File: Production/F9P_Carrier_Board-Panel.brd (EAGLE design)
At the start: 155.7 x 146.3 mm, 666 parts, among them J11 MICROMOD-2222-C, J13 U.FL, J14 QWIIC_RIGHT_ANGLE, J17 JTAG, J20 MICROMOD-2222-C, J22 U.FL, J23 QWIIC_RIGHT_ANGLE, J26 JTAG, J29 MICROMOD-2222-C, J31 U.FL, J32 QWIIC_RIGHT_ANGLE, J35 JTAG, J4 U.FL, J5 QWIIC_RIGHT_ANGLE, J6 MICROMOD-2222-C, J8 JTAG, U1 U-BLOX_ZED-F9P, U2 AP7361C-33, U3 U-BLOX_ZED-F9P, U4 AP7361C-33, U5 AP7361C-33, U6 U-BLOX_ZED-F9P, U7 AP7361C-33, U8 U-BLOX_ZED-F9P

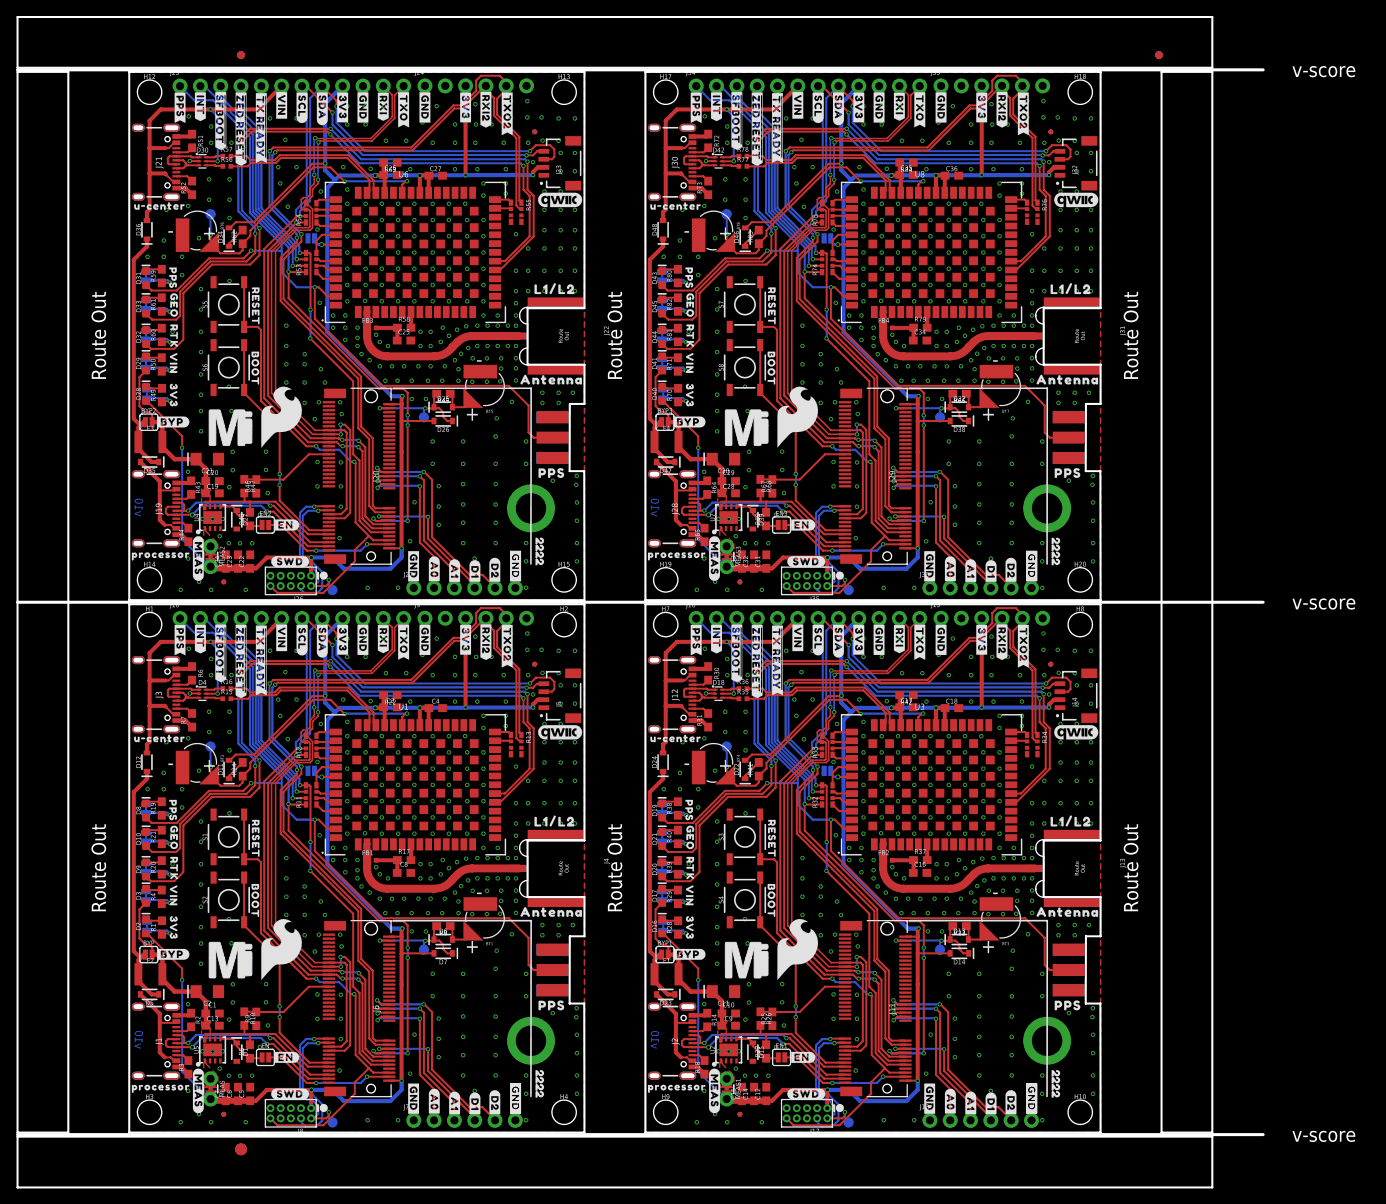
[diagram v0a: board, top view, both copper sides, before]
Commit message: Updated panel
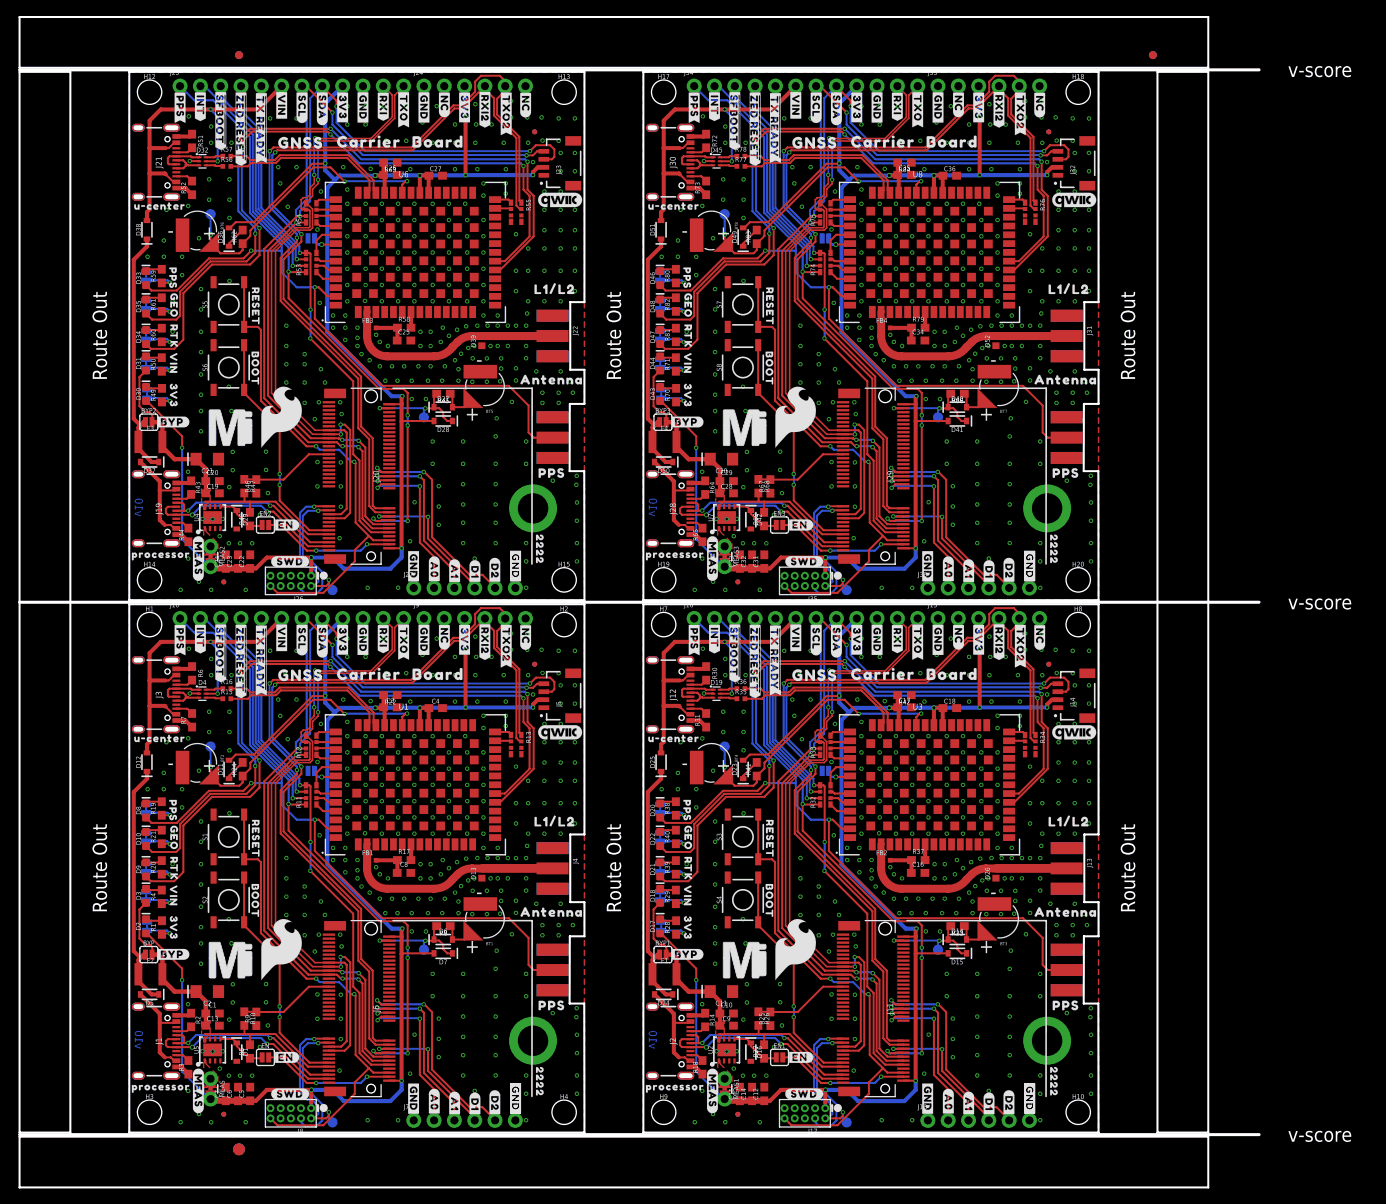
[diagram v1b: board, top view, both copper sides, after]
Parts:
- added D49: 0.5A/40V/420mV, SparkFun-DiscreteSemi:SOD-323
- added D50, D51: 3A/10V/280mV, SparkFun-DiscreteSemi:SOD-323
- added D52: PESD0402, SparkFun-DiscreteSemi:0402
- added U$329: (no value), bot:##SFBOOT##8
- added U$330: (no value), SparkFun-MicroMod:MICROMOD_LOGO_.5
- added U$331: (no value), SparkFun-MicroMod:MICROMOD_MI_LOGO_1
- added U$332: (no value), SparkFun-Aesthetics:SFE_LOGO_FLAME_.3
- added U$333, U$334, U$335, U$346, U$347: (no value), top:#GND#0
- added U$336: (no value), top:#A0#8
- added U$337: (no value), top:#A1#8
- added U$338: (no value), top:#D1#8
- added U$339: (no value), top:#D2#8
- added U$340, U$341: (no value), top:PROCESSOR23
- added U$342: (no value), bot:#A0#14
- added U$343: (no value), bot:#A1#14
- added U$344: (no value), bot:#D1#14
- added U$345: (no value), bot:#D2#14
- added U$348: (no value), top:GNSS21
- added U$349: (no value), top:GNSS501
- added U$350: (no value), top:CARRIER502
- added U$351: (no value), top:BOARD503
- added U$352: (no value), top:2222501
- added U$353, U$354: (no value), top:#NC#4
- added U$355, U$356: (no value), top:#NC#5
- D13: value 3A/10V/280mV -> PESD0402; device SparkFun-DiscreteSemi:SOD-323 -> SparkFun-DiscreteSemi:0402
- D14, D38: value 1A/23V/620mV -> 3A/10V/280mV
- D15: value 3.3V -> 1A/23V/620mV
- D16, D29: value RED -> 3.3V; device SparkFun-LED:LED-0603 -> SparkFun-DiscreteSemi:SOD-323
- D18, D30: value PRTR5V0U2F -> RED; device SparkFun-IC-Power:SOT886 -> SparkFun-LED:LED-0603
- D19, D32, D45: value BLUE -> PRTR5V0U2F; device SparkFun-LED:LED-0603 -> SparkFun-IC-Power:SOT886
- D22, D34, D46: value 0.5A/40V/420mV -> BLUE; device SparkFun-DiscreteSemi:SOD-323 -> SparkFun-LED:LED-0603
- D23, D36: value 3A/10V/280mV -> 0.5A/40V/420mV
- D26: value 1A/23V/620mV -> PESD0402; device SparkFun-DiscreteSemi:SOD-323 -> SparkFun-DiscreteSemi:0402
- D27: value 3.3V -> 3A/10V/280mV
- D28, D41: value RED -> 1A/23V/620mV; device SparkFun-LED:LED-0603 -> SparkFun-DiscreteSemi:SOD-323
- D31, D43, D44: value BLUE -> RED
- D35, D47, D48: value 3A/10V/280mV -> BLUE; device SparkFun-DiscreteSemi:SOD-323 -> SparkFun-LED:LED-0603
- D39: value 3.3V -> PESD0402; device SparkFun-DiscreteSemi:SOD-323 -> SparkFun-DiscreteSemi:0402
- D40: value RED -> 3A/10V/280mV; device SparkFun-LED:LED-0603 -> SparkFun-DiscreteSemi:SOD-323
- D42: value PRTR5V0U2F -> 3.3V; device SparkFun-IC-Power:SOT886 -> SparkFun-DiscreteSemi:SOD-323
- H11, H16, H5, H6: value STAND-OFF-REFLOW2.5MM_TALL -> STAND-OFF-REFLOW-M2.5_2.5MM_TALL
- J13, J22, J31, J4: device SparkFun-RF:SMA-EDGE-SMD -> SparkFun-RF:SMA-EDGE
- MEAS, MEAS1, MEAS2, MEAS3: value (none) -> JUMPER-COMBO_2_NC_TRACE
- U$100: device top:GEO15 -> top:#GND#0
- U$101: device top:PPS14 -> top:#GND#0
- U$102: device top:RTK16 -> top:#PPS#6
- U$103: device bot:#GEO#9 -> top:#RXI2#9
- U$104: device bot:#PPS#10 -> top:#TXO2#9
- U$105: device bot:#RTK#8 -> top:#VIN#13
- U$106: device bot:#SPI#11 -> top:GEO15
- U$107: device top:#3V3#1 -> top:PPS14
- U$108: device top:#3V3#1 -> top:RTK16
- U$109: device top:#GND#0 -> bot:#GEO#9
- U$110: device top:#GND#0 -> bot:#PPS#10
- U$111: device top:#VIN#13 -> bot:#RTK#8
- U$112: device top:#INT#10 -> bot:#SPI#11
- U$113, U$281: device top:##TX_READY##13 -> top:#3V3#1
- U$114: device bot:##TX_READY##7 -> top:#3V3#1
- U$115, U$283: device bot:#INT#4 -> top:#GND#0
- U$116: device bot:#PPS#3 -> top:#GND#0
- U$117: device bot:#TXO2#10 -> top:#VIN#13
- U$118: device bot:#RXI2#10 -> top:#INT#10
- U$119: device top:ZED#F9P19 -> top:##TX_READY##13
- U$120: device top:U#CENTER20 -> bot:##TX_READY##7
- U$121: device SparkFun-Aesthetics:QWIIC_5.5MM -> bot:#INT#4
- U$122: device bot:#SCL#1 -> bot:#PPS#3
- U$123: device bot:#SDA#0 -> bot:#TXO2#10
- U$124: device bot:#TXO#5 -> bot:#RXI2#10
- U$125: device bot:#RXI#6 -> top:ZED#F9P19
- U$126: device top:PPS15 -> top:U#CENTER20
- U$127: device top:ANTENNA16 -> SparkFun-Aesthetics:QWIIC_5.5MM
- U$128: device top:L1#L216 -> bot:#SCL#1
- U$129: device top:##CS##9 -> bot:#SDA#0
- U$130: device top:#CLK#7 -> bot:#TXO#5
- U$135: device top:#SDO#9 -> bot:#RXI#6
- U$136: device top:#SDI#11 -> top:PPS15
- U$137: device top:BLUETOOTH24 -> top:ANTENNA16
- U$138: device top:U#CENTER22 -> top:L1#L216
- U$139: device top:L1#L217 -> top:##CS##9
- U$140: device top:ANTENNA17 -> top:#CLK#7
- U$141: device top:PPS16 -> top:#SDO#9
- U$142: device bot:##ZED_RESET##9 -> top:#SDI#11
- U$143: device top:##ZED_RESET##14 -> top:BLUETOOTH24
- U$144: device top:##SFBOOT##13 -> top:U#CENTER22
- U$145: device bot:##SFBOOT##8 -> top:L1#L217
- U$146: device SparkFun-MicroMod:MICROMOD_LOGO_.5 -> top:ANTENNA17
- U$147: device SparkFun-MicroMod:MICROMOD_MI_LOGO_1 -> top:PPS16
- U$148: device SparkFun-Aesthetics:SFE_LOGO_FLAME_.3 -> bot:##ZED_RESET##9
- U$149, U$327: device top:#GND#0 -> top:##ZED_RESET##14
- U$150: device top:#GND#0 -> top:##SFBOOT##13
- U$151: device top:#GND#0 -> bot:##SFBOOT##8
- U$152: device top:#A0#8 -> SparkFun-MicroMod:MICROMOD_LOGO_.5
- U$153: device top:#A1#8 -> SparkFun-MicroMod:MICROMOD_MI_LOGO_1
- U$154: device top:#D1#8 -> SparkFun-Aesthetics:SFE_LOGO_FLAME_.3
- U$155: device top:#D2#8 -> top:#GND#0
- U$156, U$157: device top:PROCESSOR23 -> top:#GND#0
- U$158: device bot:#A0#14 -> top:#A0#8
- U$159: device bot:#A1#14 -> top:#A1#8
- U$160: device bot:#D1#14 -> top:#D1#8
- U$161: device bot:#D2#14 -> top:#D2#8
- U$162, U$163: device top:#GND#0 -> top:PROCESSOR23
- U$164: device top:GNSS21 -> bot:#A0#14
- U$165: device buzzard_labels (9):22229 -> bot:#A1#14
- U$166: device power:#BYP#8 -> bot:#D1#14
- U$167: device power:#RESET10 -> bot:#D2#14
- U$168: device power:BOOT10 -> top:#GND#0
- U$169: device power:#MEAS#10 -> top:#GND#0
- U$170: device power:#SWD#10 -> top:GNSS21
- U$171: device headers_dup:VIN3 -> top:GNSS501
- U$172: device headers_dup:3V34 -> top:CARRIER502
- U$173: device fl3:#SWD#10 -> top:BOARD503
- U$174: device fl3:#MEAS#10 -> top:2222501
- U$175: device fl3:#VIN_LED#10 -> top:#NC#4
- U$176: device fl3:#3V3_LED#10 -> top:#NC#4
- U$177: device output:#EN#0 -> top:#NC#5
- U$178: device top:#3V3#1 -> top:#NC#5
- U$179: device top:#3V3#1 -> power:#BYP#8
- U$180: device top:#GND#0 -> power:#RESET10
- U$181: device top:#GND#0 -> power:BOOT10
- U$182: device top:#PPS#6 -> power:#MEAS#10
- U$183: device top:#RXI2#9 -> power:#SWD#10
- U$184: device top:#TXO2#9 -> headers_dup:VIN3
- U$185: device top:#VIN#13 -> headers_dup:3V34
- U$186: device top:GEO15 -> fl3:#SWD#10
- U$187: device top:PPS14 -> fl3:#MEAS#10
- U$188: device top:RTK16 -> fl3:#VIN_LED#10
- U$189: device bot:#GEO#9 -> fl3:#3V3_LED#10
- U$190: device bot:#PPS#10 -> output:#EN#0
- U$191: device bot:#RTK#8 -> top:#3V3#1
- U$192: device bot:#SPI#11 -> top:#3V3#1
- U$193, U$194: device top:#3V3#1 -> top:#GND#0
- U$195: device top:#GND#0 -> top:#PPS#6
- U$196: device top:#GND#0 -> top:#RXI2#9
- U$197: device top:#VIN#13 -> top:#TXO2#9
- U$198: device top:#INT#10 -> top:#VIN#13
- U$199: device top:##TX_READY##13 -> top:GEO15
- U$200: device bot:##TX_READY##7 -> top:PPS14
- U$201: device bot:#INT#4 -> top:RTK16
- U$202: device bot:#PPS#3 -> bot:#GEO#9
- U$203: device bot:#TXO2#10 -> bot:#PPS#10
- U$204: device bot:#RXI2#10 -> bot:#RTK#8
- U$205: device top:ZED#F9P19 -> bot:#SPI#11
- U$206: device top:U#CENTER20 -> top:#3V3#1
- U$207: device SparkFun-Aesthetics:QWIIC_5.5MM -> top:#3V3#1
- U$208: device bot:#SCL#1 -> top:#GND#0
- U$209: device bot:#SDA#0 -> top:#GND#0
- U$210: device bot:#TXO#5 -> top:#VIN#13
- U$211: device bot:#RXI#6 -> top:#INT#10
- U$212: device top:PPS15 -> top:##TX_READY##13
- U$213: device top:ANTENNA16 -> bot:##TX_READY##7
- U$214: device top:L1#L216 -> bot:#INT#4
- U$215: device top:##CS##9 -> bot:#PPS#3
- U$216: device top:#CLK#7 -> bot:#TXO2#10
- U$217: device top:#SDO#9 -> bot:#RXI2#10
- U$218: device top:#SDI#11 -> top:ZED#F9P19
- U$219: device top:BLUETOOTH24 -> top:U#CENTER20
- U$220: device top:U#CENTER22 -> SparkFun-Aesthetics:QWIIC_5.5MM
- U$221: device top:L1#L217 -> bot:#SCL#1
- U$222: device top:ANTENNA17 -> bot:#SDA#0
- U$223: device top:PPS16 -> bot:#TXO#5
- U$224: device bot:##ZED_RESET##9 -> bot:#RXI#6
- U$225: device top:##ZED_RESET##14 -> top:PPS15
- U$226: device top:##SFBOOT##13 -> top:ANTENNA16
- U$227: device bot:##SFBOOT##8 -> top:L1#L216
- U$228: device SparkFun-MicroMod:MICROMOD_LOGO_.5 -> top:##CS##9
- U$229: device SparkFun-MicroMod:MICROMOD_MI_LOGO_1 -> top:#CLK#7
- U$230: device SparkFun-Aesthetics:SFE_LOGO_FLAME_.3 -> top:#SDO#9
- U$231: device top:#GND#0 -> top:#SDI#11
- U$232: device top:#GND#0 -> top:BLUETOOTH24
- U$233: device top:#GND#0 -> top:U#CENTER22
- U$234: device top:#A0#8 -> top:L1#L217
- U$235: device top:#A1#8 -> top:ANTENNA17
- U$236: device top:#D1#8 -> top:PPS16
- U$237: device top:#D2#8 -> bot:##ZED_RESET##9
- U$238: device top:PROCESSOR23 -> top:##ZED_RESET##14
- U$239: device top:PROCESSOR23 -> top:##SFBOOT##13
- U$240: device bot:#A0#14 -> bot:##SFBOOT##8
- U$241: device bot:#A1#14 -> SparkFun-MicroMod:MICROMOD_LOGO_.5
- U$242: device bot:#D1#14 -> SparkFun-MicroMod:MICROMOD_MI_LOGO_1
- U$243: device bot:#D2#14 -> SparkFun-Aesthetics:SFE_LOGO_FLAME_.3
- U$246: device top:GNSS21 -> top:#GND#0
- U$247: device buzzard_labels (9):22229 -> top:#A0#8
- U$248: device power:#BYP#8 -> top:#A1#8
- U$249: device power:#RESET10 -> top:#D1#8
- U$250: device power:BOOT10 -> top:#D2#8
- U$251: device power:#MEAS#10 -> top:PROCESSOR23
- U$252: device power:#SWD#10 -> top:PROCESSOR23
- U$253: device headers_dup:VIN3 -> bot:#A0#14
- U$254: device headers_dup:3V34 -> bot:#A1#14
- U$255: device fl3:#SWD#10 -> bot:#D1#14
- U$256: device fl3:#MEAS#10 -> bot:#D2#14
- U$257: device fl3:#VIN_LED#10 -> top:#GND#0
- U$258: device fl3:#3V3_LED#10 -> top:#GND#0
- U$259: device output:#EN#0 -> top:GNSS21
- U$260: device top:#3V3#1 -> top:GNSS501
- U$261: device top:#3V3#1 -> top:CARRIER502
- U$262: device top:#GND#0 -> top:BOARD503
- U$263: device top:#GND#0 -> top:2222501
- U$264: device top:#PPS#6 -> top:#NC#4
- U$265: device top:#RXI2#9 -> top:#NC#4
- U$266: device top:#TXO2#9 -> top:#NC#5
- U$267: device top:#VIN#13 -> top:#NC#5
- U$268: device top:GEO15 -> power:#BYP#8
- U$269: device top:PPS14 -> power:#RESET10
- U$270: device top:RTK16 -> power:BOOT10
- U$271: device bot:#GEO#9 -> power:#MEAS#10
- U$272: device bot:#PPS#10 -> power:#SWD#10
- U$273: device bot:#RTK#8 -> headers_dup:VIN3
- U$274: device bot:#SPI#11 -> headers_dup:3V34
- U$275, U$93: device top:#3V3#1 -> fl3:#SWD#10
- U$276: device top:#3V3#1 -> fl3:#MEAS#10
- U$277, U$95: device top:#GND#0 -> fl3:#VIN_LED#10
- U$278: device top:#GND#0 -> fl3:#3V3_LED#10
- U$279: device top:#VIN#13 -> output:#EN#0
- U$280: device top:#INT#10 -> top:#3V3#1
- U$282: device bot:##TX_READY##7 -> top:#GND#0
- U$284: device bot:#PPS#3 -> top:#PPS#6
- U$285: device bot:#TXO2#10 -> top:#RXI2#9
- U$286: device bot:#RXI2#10 -> top:#TXO2#9
- U$287: device top:ZED#F9P19 -> top:#VIN#13
- U$288: device top:U#CENTER20 -> top:GEO15
- U$289: device SparkFun-Aesthetics:QWIIC_5.5MM -> top:PPS14
- U$290: device bot:#SCL#1 -> top:RTK16
- U$291: device bot:#SDA#0 -> bot:#GEO#9
- U$292: device bot:#TXO#5 -> bot:#PPS#10
- U$293: device bot:#RXI#6 -> bot:#RTK#8
- U$294: device top:PPS15 -> bot:#SPI#11
- U$295: device top:ANTENNA16 -> top:#3V3#1
- U$296: device top:L1#L216 -> top:#3V3#1
- U$297: device top:##CS##9 -> top:#GND#0
- U$298: device top:#CLK#7 -> top:#GND#0
- U$299: device top:#SDO#9 -> top:#VIN#13
- U$300: device top:#SDI#11 -> top:#INT#10
- U$301: device top:BLUETOOTH24 -> top:##TX_READY##13
- U$302: device top:U#CENTER22 -> bot:##TX_READY##7
- U$303: device top:L1#L217 -> bot:#INT#4
- U$304: device top:ANTENNA17 -> bot:#PPS#3
- U$305: device top:PPS16 -> bot:#TXO2#10
- U$306: device bot:##ZED_RESET##9 -> bot:#RXI2#10
- U$307: device top:##ZED_RESET##14 -> top:ZED#F9P19
- U$308: device top:##SFBOOT##13 -> top:U#CENTER20
- U$309: device bot:##SFBOOT##8 -> SparkFun-Aesthetics:QWIIC_5.5MM
- U$310: device SparkFun-MicroMod:MICROMOD_LOGO_.5 -> bot:#SCL#1
- U$311: device SparkFun-MicroMod:MICROMOD_MI_LOGO_1 -> bot:#SDA#0
- U$312: device SparkFun-Aesthetics:SFE_LOGO_FLAME_.3 -> bot:#TXO#5
- U$313: device top:#GND#0 -> bot:#RXI#6
- U$314: device top:#GND#0 -> top:PPS15
- U$315: device top:#GND#0 -> top:ANTENNA16
- U$316: device top:#A0#8 -> top:L1#L216
- U$317: device top:#A1#8 -> top:##CS##9
- U$318: device top:#D1#8 -> top:#CLK#7
- U$319: device top:#D2#8 -> top:#SDO#9
- U$320: device top:PROCESSOR23 -> top:#SDI#11
- U$321: device top:PROCESSOR23 -> top:BLUETOOTH24
- U$322: device bot:#A0#14 -> top:U#CENTER22
- U$323: device bot:#A1#14 -> top:L1#L217
- U$324: device bot:#D1#14 -> top:ANTENNA17
- U$325: device bot:#D2#14 -> top:PPS16
- U$326: device top:#GND#0 -> bot:##ZED_RESET##9
- U$328: device top:GNSS21 -> top:##SFBOOT##13
- U$55: device buzzard_labels (9):22229 -> top:#NC#4
- U$79: device buzzard_labels (9):22229 -> top:GNSS501
- U$80: device power:#BYP#8 -> top:CARRIER502
- U$81: device power:#RESET10 -> top:BOARD503
- U$82: device power:BOOT10 -> top:2222501
- U$83: device power:#MEAS#10 -> top:#NC#4
- U$84: device power:#SWD#10 -> top:#NC#5
- U$85: device headers_dup:VIN3 -> top:#NC#5
- U$86: device headers_dup:3V34 -> power:#BYP#8
- U$87: device fl3:#SWD#10 -> power:#RESET10
- U$88: device fl3:#MEAS#10 -> power:BOOT10
- U$89: device fl3:#VIN_LED#10 -> power:#MEAS#10
- U$90: device fl3:#3V3_LED#10 -> power:#SWD#10
- U$91: device output:#EN#0 -> headers_dup:VIN3
- U$92: device top:#3V3#1 -> headers_dup:3V34
- U$94: device top:#GND#0 -> fl3:#MEAS#10
- U$96: device top:#PPS#6 -> fl3:#3V3_LED#10
- U$97: device top:#RXI2#9 -> output:#EN#0
- U$98: device top:#TXO2#9 -> top:#3V3#1
- U$99: device top:#VIN#13 -> top:#3V3#1
- moved U$167 137.0 mm to (110.0, 3.63), flipped to the bottom, turned to 90 degrees
- moved U$166 133.1 mm to (107.5, 3.48), flipped to the bottom, turned to 90 degrees
- moved U$168 133.0 mm to (112.5, 4.24), flipped to the bottom, turned to 90 degrees
- moved U$174 125.4 mm to (115.6, 6.35), flipped to the top, turned to 270 degrees
- moved U$169 123.9 mm to (112.5, 4.24)
- moved U$176 111.4 mm to (113.8, 62.0), flipped to the top, turned to 270 degrees
- moved U$79 106.0 mm to (21.5, 57.1), turned to 0 degrees
- moved D38 104.3 mm to (2.21, 112.9), turned to 90 degrees
- moved U$175 103.1 mm to (103.7, 62.1), flipped to the top, turned to 270 degrees
- moved D37 101.5 mm to (2.54, 83.8), turned to 180 degrees
- moved U$178 97.6 mm to (113.8, 62.0)
- moved U$172 95.3 mm to (94.2, 57.3), turned to 0 degrees
- moved U$170 90.8 mm to (99.8, 27.9), flipped to the bottom
- moved U$165 89.6 mm to (104.9, 3.53), flipped to the bottom, turned to 90 degrees
- moved D26 89.3 mm to (108.3, 32.4), turned to 90 degrees
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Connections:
- net 3.3V1: now also D15.A, D17.A, D23.A; no longer D14.A, D16.A, D22.A
- net 3.3V2: now also D30.A, D36.A; no longer D26.A, D34.A
- net 3.3V3: now also D41.A, D43.A, D49.A; no longer D38.A, D40.A, D46.A
- net 3.3V_EN1: now also D16.C; no longer D15.C
- net 3.3V_EN2: now also D29.C; no longer D27.C
- net 3.3V_EN3: now also D42.C; no longer D39.C
- net GEO_STAT1: now also D22.A; no longer D21.A
- net GEO_STAT2: now also D35.A; no longer D33.A
- net GEO_STAT3: now also D48.A; no longer D45.A
- net GND: now also D13.1, J4.GND@2, J4.GND@3
- net GND1: now also D16.A, D19.2, D26.1, J13.GND@2, J13.GND@3; no longer D15.A, D18.2
- net GND2: now also D29.A, D32.2, D39.1, J22.GND@2, J22.GND@3; no longer D27.A, D30.2
- net GND3: now also D42.A, D45.2, D52.1, J31.GND@2, J31.GND@3; no longer D39.A, D42.2
- net N$103: now also D45.3; no longer D42.3
- net N$104: now also D45.1; no longer D42.1
- net N$110: now also D46.C; no longer D43.C
- net N$111: now also D47.C; no longer D44.C
- net N$113: now also D48.C; no longer D45.C
- net N$114: now also D49.C; no longer D46.C
- net N$115: now also D43.C; no longer D40.C
- net N$118: now also D44.C; no longer D41.C
- net N$127: now also D45.6; no longer D42.6
- net N$128: now also D45.4; no longer D42.4
- net N$33: now also D14.A; no longer D13.A
- net N$37: now also D19.3; no longer D18.3
- net N$38: now also D19.1; no longer D18.1
- net N$44: now also D20.C; no longer D19.C
- net N$47: now also D21.C; no longer D20.C
- net N$49: now also D22.C; no longer D21.C
- net N$50: now also D23.C; no longer D22.C
- net N$51: now also D17.C; no longer D16.C
- net N$54: now also D18.C; no longer D17.C
- net N$63: now also D19.6; no longer D18.6
- net N$64: now also D19.4; no longer D18.4
- net N$67: now also D27.A; no longer D25.A
- net N$71: now also D32.3; no longer D30.3
- net N$72: now also D32.1; no longer D30.1
- net N$78: now also D33.C; no longer D31.C
- net N$79: now also D34.C; no longer D32.C
- net N$81: now also D35.C; no longer D33.C
- net N$82: now also D36.C; no longer D34.C
- net N$83: now also D30.C; no longer D28.C
- net N$86: now also D31.C; no longer D29.C
- net N$95: now also D32.6; no longer D30.6
- net N$96: now also D32.4; no longer D30.4
- net N$99: now also D40.A; no longer D37.A
- net PPS1: now also D20.A; no longer D19.A
- net PPS2: now also D33.A; no longer D31.A
- net PPS3: now also D46.A; no longer D43.A
- net RF_IN: now also D13.2
- net RF_IN1: now also D26.2
- net RF_IN2: now also D39.2
- net RF_IN3: now also D52.2
- net RTC_3V: now also TP1.1; no longer TP1.P$1
- net RTC_3V1: now also D15.C, TP4.1; no longer D13.C, TP4.P$1
- net RTC_3V2: now also D27.C, D28.C, TP7.1; no longer D25.C, D26.C, TP7.P$1
- net RTC_3V3: now also D40.C, D41.C, TP10.1; no longer D37.C, D38.C, TP10.P$1
- net RTK_STAT1: now also D21.A; no longer D20.A
- net RTK_STAT2: now also D34.A; no longer D32.A
- net RTK_STAT3: now also D47.A; no longer D44.A
- net SWDIO: now also TP2.1; no longer TP2.P$1
- net SWDIO1: now also TP5.1; no longer TP5.P$1
- net SWDIO2: now also TP8.1; no longer TP8.P$1
- net SWDIO3: now also TP11.1; no longer TP11.P$1
- net VIN1: now also D18.A; no longer D17.A
- net VIN2: now also D31.A; no longer D29.A
- net VIN3: now also D44.A; no longer D41.A
- net V_BATT: now also TP3.1; no longer TP3.P$1
- net V_BATT1: now also TP6.1; no longer TP6.P$1
- net V_BATT2: now also TP9.1; no longer TP9.P$1
- net V_BATT3: now also TP12.1; no longer TP12.P$1
- net V_FUSE1: now also D25.C; no longer D23.C
- net V_FUSE2: now also D37.C, D38.C; no longer D35.C, D36.C
- net V_FUSE3: now also D50.C, D51.C; no longer D47.C, D48.C
- net V_USB1: now also D24.A; no longer D23.A
- net V_USB2: now also D37.A; no longer D35.A
- net V_USB3: now also D50.A; no longer D47.A
- net V_USB_1: now also D19.5, D25.A; no longer D18.5, D24.A
- net V_USB_3: now also D32.5, D38.A; no longer D30.5, D36.A
- net V_USB_4: now also D45.5, D51.A; no longer D42.5, D48.A
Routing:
- net RF_IN2: track 22.5 -> 35.5 mm
- net RF_IN: track 22.5 -> 35.5 mm
- net RF_IN3: track 22.5 -> 35.5 mm
- net RF_IN1: track 22.5 -> 35.5 mm
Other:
- board size 155.7 x 146.3 mm -> 154.9 x 146.3 mm
